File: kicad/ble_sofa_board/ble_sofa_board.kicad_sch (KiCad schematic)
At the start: 4 parts

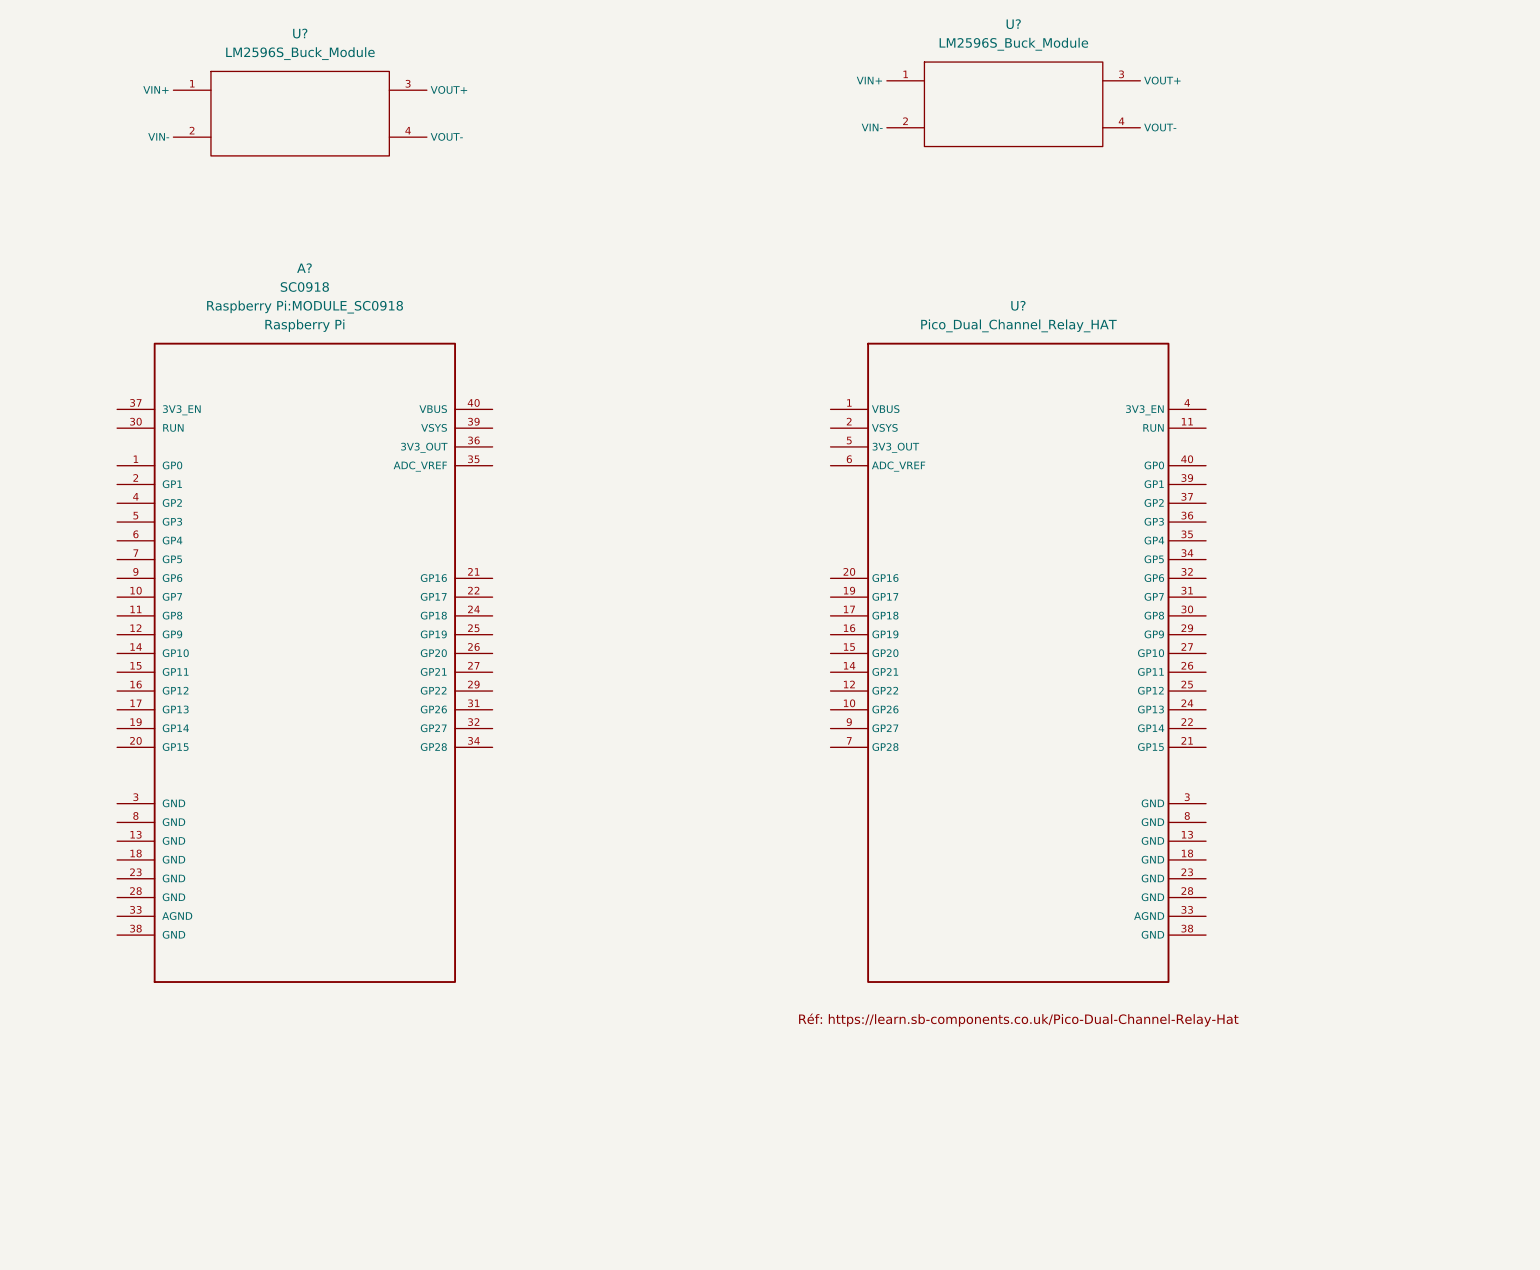
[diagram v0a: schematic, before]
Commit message: ble_sofa_board - WIP schematic
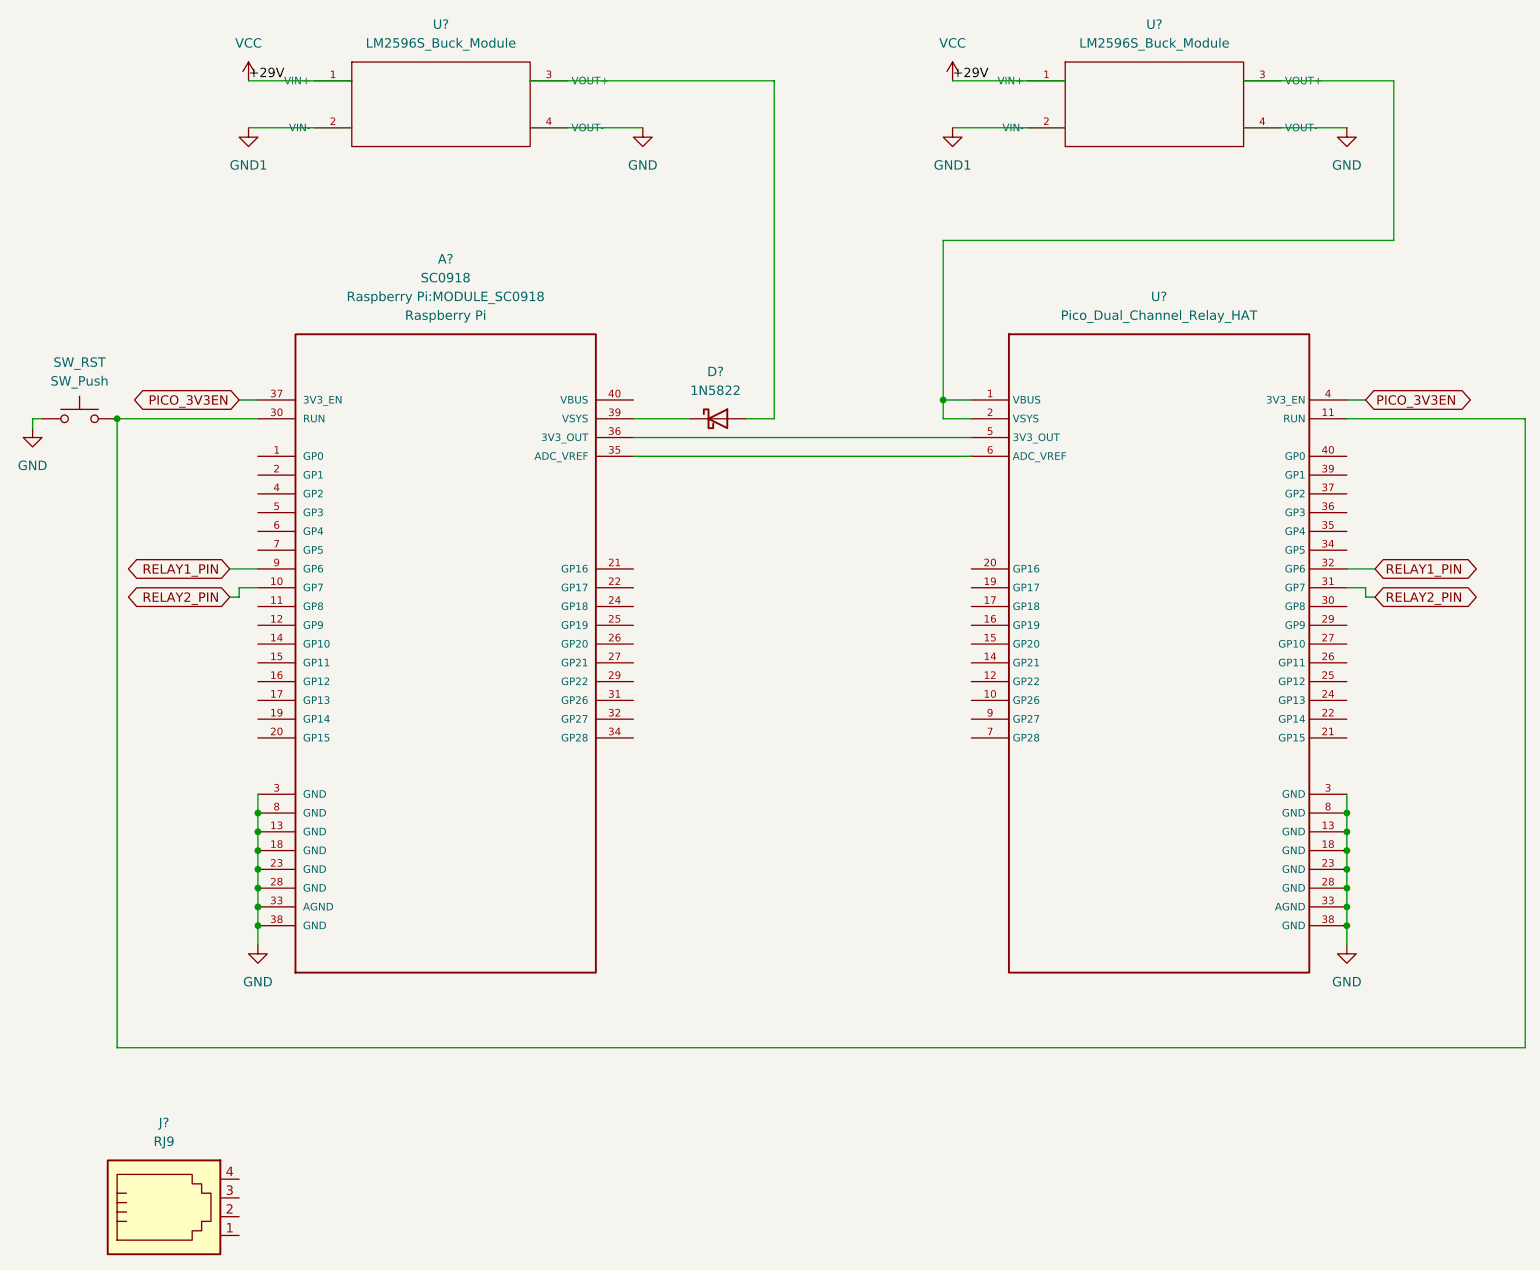
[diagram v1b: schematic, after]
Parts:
- added D?: 1N5822, Diode_THT:D_DO-201AD_P15.24mm_Horizontal, symbol Diode:1N5822
- added J?: RJ9, symbol Connector:RJ9
- added SW_RST: SW_Push, symbol Switch:SW_Push
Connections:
- net RELAY2_PIN: now reaches A?.10 (GP7)
- net RELAY2_PIN: now also U?.31 (GP7)
- net GND: now reaches A?.13 (GND)
- net GND: now also A?.18 (GND), A?.23 (GND), A?.28 (GND), A?.3 (GND), A?.33 (AGND), A?.38 (GND), A?.8 (GND), U?.13 (GND), U?.18 (GND), U?.23 (GND), U?.28 (GND), U?.3 (GND), U?.33 (AGND), U?.38 (GND), U?.4 (VOUT-), U?.4 (VOUT-), U?.8 (GND), SW_RST.1
- net at A?.30 (RUN): now also U?.11 (RUN), SW_RST.2
- net at A?.35 (ADC_VREF): now also U?.6 (ADC_VREF)
- net at A?.36 (3V3_OUT): now also U?.5 (3V3_OUT)
- net PICO_3V3EN: now reaches A?.37 (3V3_EN)
- net PICO_3V3EN: now also U?.4 (3V3_EN)
- net at A?.39 (VSYS): now also D?.1 (K)
- net RELAY1_PIN: now reaches A?.9 (GP6)
- net RELAY1_PIN: now also U?.32 (GP6)
- net at U?.1 (VBUS): now also U?.2 (VSYS), U?.3 (VOUT+)
- net VCC: now reaches U?.1 (VIN+)
- net VCC: now also U?.1 (VIN+)
- net GND1: now reaches U?.2 (VIN-)
- net GND1: now also U?.2 (VIN-)
- net at U?.3 (VOUT+): now also D?.2 (A)
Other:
- title: (none) -> BLE Sofa Board
- moved on the sheet: A?, U?
